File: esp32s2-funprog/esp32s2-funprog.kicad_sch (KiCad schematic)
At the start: 70 parts, among them J1 OPGM, J2 PGM, J3 USB_C_Receptacle_USB2.0, J4 MOUNT, J5 MOUNT, Q1 SE4625-PandN, Q2 SE4625-PandN, Q3 DWL336C, Q4 MOT2302, Q5 MOT2302, SW1 TS-1187A-B-A-B, U1 ESP32-S2, U2 AP1117-33, U3 MT3608, U4 LM321, U5 ZDT6790TA, U6 COS4514, U8 HP3000, Y1 40MHz

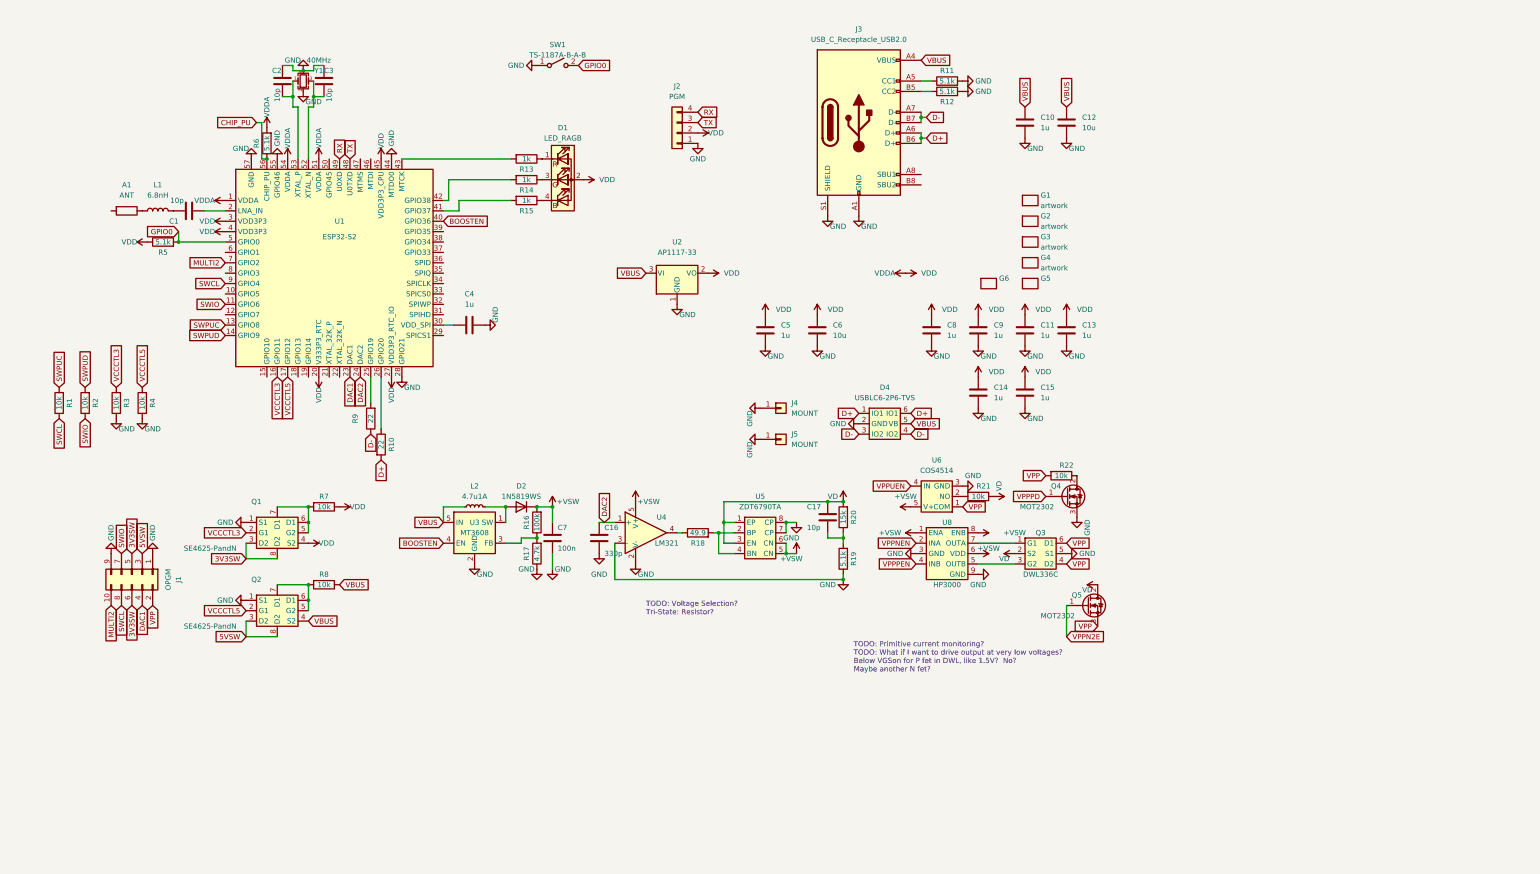
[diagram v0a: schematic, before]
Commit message: update with rev
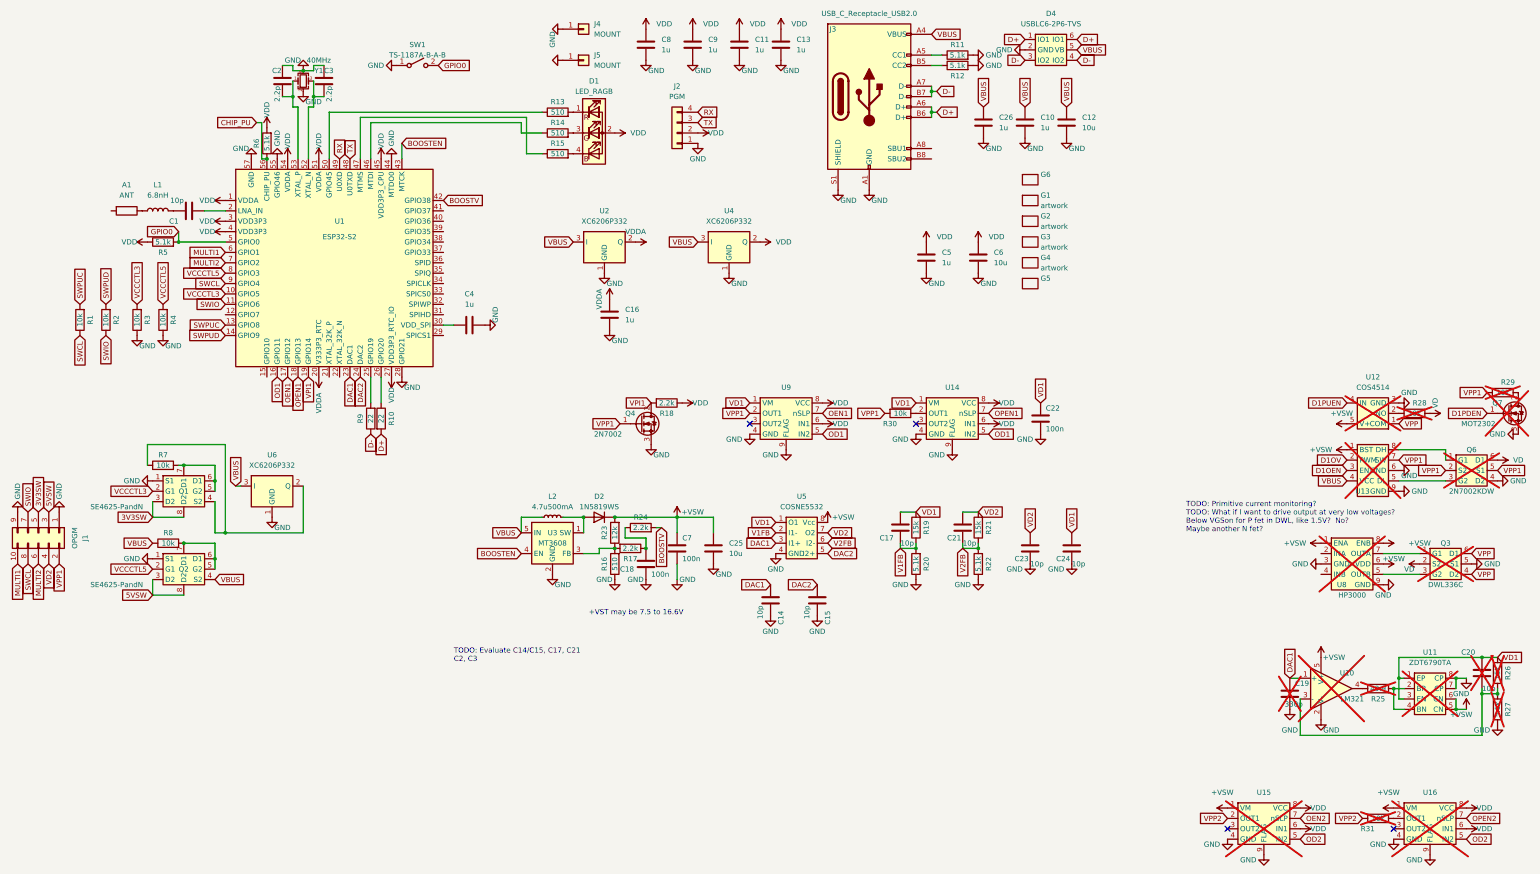
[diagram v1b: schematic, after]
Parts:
- removed Q5: MOT2302, Package_TO_SOT_SMD:SOT-23, symbol Device:Q_NMOS_GDS
- removed U2: AP1117-33, Package_TO_SOT_SMD:SOT-223-3_TabPin2, symbol Regulator_Linear:AP1117-33
- removed U4: LM321, Package_TO_SOT_SMD:SOT-23-5, symbol Amplifier_Operational:LM321
- removed U5: ZDT6790TA, Package_TO_SOT_SMD:SOT-223-8, symbol cnhardware:ZDT6790-COMPLEMENTARY-BJT
- removed U6: COS4514, Package_TO_SOT_SMD:SOT-23-5, symbol cnhardware:COS4514-MUX-SPST
- added C18, C22: 100n, Capacitor_SMD:C_0402_1005Metric, symbol Device:C
- added C19: 330p, Capacitor_SMD:C_0402_1005Metric, symbol Device:C
- added C20, C21, C23, C24: 10p, Capacitor_SMD:C_0402_1005Metric, symbol Device:C
- added C25: 10u, Capacitor_SMD:C_0603_1608Metric, symbol Device:C
- added C26: 1u, Capacitor_SMD:C_0402_1005Metric, symbol Device:C
- added Q6: 2N7002KDW, Package_TO_SOT_SMD:SOT-363_SC-70-6, symbol cnhardware:DWL336C-P-AND-N
- added Q7: MOT2302, Package_TO_SOT_SMD:SOT-23, symbol Device:Q_NMOS_GDS
- added R23: 12k, Resistor_SMD:R_0402_1005Metric, symbol Device:R
- added R24: 2.2k, Resistor_SMD:R_0402_1005Metric, symbol Device:R
- added R25: 49.9, Resistor_SMD:R_0402_1005Metric, symbol Device:R
- added R26: 15k, Resistor_SMD:R_0402_1005Metric, symbol Device:R
- added R27: 5.1k, Resistor_SMD:R_0402_1005Metric, symbol Device:R
- added R28, R29, R30, R31: 10k, Resistor_SMD:R_0402_1005Metric, symbol Device:R
- added U10: LM321, Package_TO_SOT_SMD:SOT-23-5, symbol Amplifier_Operational:LM321
- added U11: ZDT6790TA, Package_TO_SOT_SMD:SOT-223-8, symbol cnhardware:ZDT6790-COMPLEMENTARY-BJT
- added U12: COS4514, Package_TO_SOT_SMD:SOT-23-5, symbol cnhardware:COS4514-MUX-SPST
- added U13: ~, Package_DFN_QFN:DFN-8-1EP_3x3mm_P0.5mm_EP1.65x2.38mm, symbol cnhardware:NCP81155-GATE-DRIVER
- added U14, U15, U16, U9: AT8837, Package_DFN_QFN:DFN-8-1EP_2x2mm_P0.45mm_EP0.64x1.38mm, symbol cnhardware:BDR6122TC-MOTOR-DRIVER
- added U2, U4, U6: XC6206P332, Package_TO_SOT_SMD:SOT-23, symbol Regulator_Linear:IFX27001TFV26
- added U5: COSNE5532, Package_SO:MSOP-8_3x3mm_P0.65mm, symbol cnhardware:LM2903-SOIC8
- C14, C15: value 1u -> 10p; LCSC C106254 -> C106199
- C16: value 330p -> 1u; LCSC C13533 -> C106254
- C2, C3: value 10p -> 2.2p; LCSC C106199 -> C1559
- L2: value 4.7u1A -> 4.7u500mA; footprint Inductor_SMD:L_1008_2520Metric -> Inductor_SMD:L_0805_2012Metric; LCSC C98340 -> C63166
- Q3, U8: now not fitted; now left out of the parts list
- Q4: value MOT2302 -> 2N7002; LCSC C5143129 -> C8545
- R13, R14, R15: value 1k -> 510; LCSC C102748 -> C25123
- R16: value 100k -> 510; LCSC C25741 -> C25123
- R17: value 4.7k -> 2.2k; LCSC C25900 -> C25879
- R18: value 49.9 -> 2.2k; LCSC C25120 -> C25879
- R19: value 5.1k -> 15k; LCSC C105872 -> C25756
- R20: value 15k -> 5.1k; LCSC C25756 -> C105872
- R21: value 10k -> 15k; LCSC C144807 -> C25756
- R22: value 10k -> 5.1k; LCSC C144807 -> C105872
- U3: footprint Package_TO_SOT_SMD:SOT-23-6 -> Package_TO_SOT_SMD:SOT-23-5
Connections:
- net +VSW: now also C25.1, R23.2, U10.5 (V+), U11.5 (CN), U11.6 (CN), U12.5 (V+), U13.1 (BST), U15.1 (VM), U16.1 (VM), U5.8 (Vcc); no longer R16.2
- net 3V3SW: no longer J1.6 (Pin_6)
- net BOOSTEN: now also U1.43 (MTCK); no longer U1.40 (GPIO36)
- net DAC1: now also C14.2, C19.1, U10.1 (+), U5.3 (I1+); no longer J1.4 (Pin_4)
- net DAC2: now also C15.2, U5.5 (I2+); no longer C16.1
- net GND: now also C14.1, C15.1, R16.1, R20.1, R22.1, C18.2, C19.2, C22.2, C23.2, C24.2, C25.2, C26.1, Q6.4 (D2), Q7.3 (S), R27.1, U10.2 (V-), U11.7 (CP), U11.8 (CP), U12.3 (GND), U13.6 (GND), U13.9 (GND), U14.4 (GND), U14.9 (FLAG), U15.4 (GND), U15.9 (FLAG), U16.4 (GND), U16.9 (FLAG), U2.1 (GND), U4.1 (GND), U5.4 (GND), U6.1 (GND), U9.4 (GND), U9.9 (FLAG); no longer C14.2, C15.2, R17.1, R19.1
- net MULTI2: now also J1.6 (Pin_6); no longer J1.10 (Pin_10)
- net VBUS: now also C26.2, U13.4 (VCC), U2.3 (I), U4.3 (I), U6.3 (I)
- net VCCCTL3: now also U1.10 (GPIO5); no longer U1.16 (GPIO11)
- net VCCCTL5: now also U1.8 (GPIO3); no longer U1.17 (GPIO12)
- net VD: now also Q6.6 (D1), R28.1; no longer C17.1, R20.2, R21.1
- net VDD: now also R18.1, U14.6 (IN1), U14.8 (VCC), U15.6 (IN1), U15.8 (VCC), U16.6 (IN1), U16.8 (VCC), U4.2 (Q), U9.6 (IN1), U9.8 (VCC); no longer C14.1, C15.1, Q1.4 (S2), R7.1, U1.20 (V333P3_RTC)
- net VPP: now also U12.1 (COM); no longer J1.2 (Pin_2), R22.2
- net VPI1: now reaches Q4.2 (D)
- net VPI1: now also R18.2, U1.19 (GPIO14); no longer R22.1
- net at R17.2, U3.3 (FB): now also R16.2, R23.1; no longer R16.1
- net VD2: now reaches R21.2
- net VD2: now also J1.4 (Pin_4), C21.1, C23.1, U5.7 (O2)
- net OPEN1: now reaches U1.18 (GPIO13)
- net OPEN1: now also U14.7 (nSLP)
- net at R15.2: now also D1.4 (BK); no longer U1.41 (GPIO37)
- net at R14.2: now also D1.3 (GK); no longer U1.42 (GPIO38)
- net at R13.2: now also D1.1 (RK); no longer U1.43 (MTCK)
- net at U1.46 (MTDI): now also R14.1
- net at U1.47 (MTMS): now also R15.1
- net at U1.50 (GPIO45): now also R13.1
- net MULTI1: now reaches U1.6 (GPIO1)
- net MULTI1: now also J1.10 (Pin_10)
- net VPPNEN: no longer names the net of U8.2 (INA)
- net VPPPD renamed VPP1
- net VPP1: now also J1.2 (Pin_2), Q6.2 (S2), Q6.5 (S1), R29.2, R30.2, U13.7 (SW), U9.2 (OUT1)
- net VPPPEN: no longer names the net of U8.4 (INB)
- new net: R30.1, U14.2 (OUT1)
- new net: Q1.4 (S2), R7.1, U6.2 (Q)
- new net: Q7.2 (D), R29.1
- new net: C20.2, R26.1, R27.2, U10.3 (-)
- new net: R31.1, U16.2 (OUT1)
- new net: R25.2, U11.2 (BP), U11.4 (BN)
- new net: R28.2, U12.2 (NO)
- new net: Q6.3 (G2), U13.5 (DL)
- new net: Q6.1 (G1), U13.8 (DH)
- new net: C18.1, R17.1, R24.1
- new net: R25.1, U10.4
- new net BOOSTV: R24.2, U1.42 (GPIO38)
- new net D1OEN: U13.3 (EN)
- new net D1OV: U13.2 (PWM)
- new net D1PDEN: Q7.1 (G)
- new net D1PUEN: U12.4 (IN)
- new net OD1: U1.16 (GPIO11), U14.5 (IN2), U9.5 (IN2)
- new net OD2: U15.5 (IN2), U16.5 (IN2)
- new net OEN1: U1.17 (GPIO12), U9.7 (nSLP)
- new net OEN2: U15.7 (nSLP)
- new net OPEN2: U16.7 (nSLP)
- new net V1FB: C17.2, R19.1, R20.2, U5.2 (I1-)
- new net V2FB: C21.2, R21.1, R22.2, U5.6 (I2-)
- new net VD1: C17.1, C20.1, C22.1, C24.1, R19.2, R26.2, U11.1 (EP), U11.3 (EN), U14.1 (VM), U5.1 (O1), U9.1 (VM)
- new net VDDA: C16.1, U1.20 (V333P3_RTC), U2.2 (Q)
- new net VPP2: R31.2, U15.2 (OUT1)
- no-connect marks 0 -> 4
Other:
- note added: "+VST may be 7.5 to 16.6V"
- note added: "TODO: Evaluate C14/C15, C17, C21 C2, C3"
- note removed: "TODO: Voltage Selection? Tri-State: Resistor?"
- moved on the sheet: C11, C13, C5, C6, C7, C8, C9, D2, D4, G6, J1, J3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
